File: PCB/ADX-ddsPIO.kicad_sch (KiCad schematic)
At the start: 72 parts, among them J1 Conn_Coaxial, J2 +12V, Q1 BS170, Q2 BS170, Q3 BS170, Q5 BS170, U1 L7805, U2 74LS244, U4 CD2003GB_GP

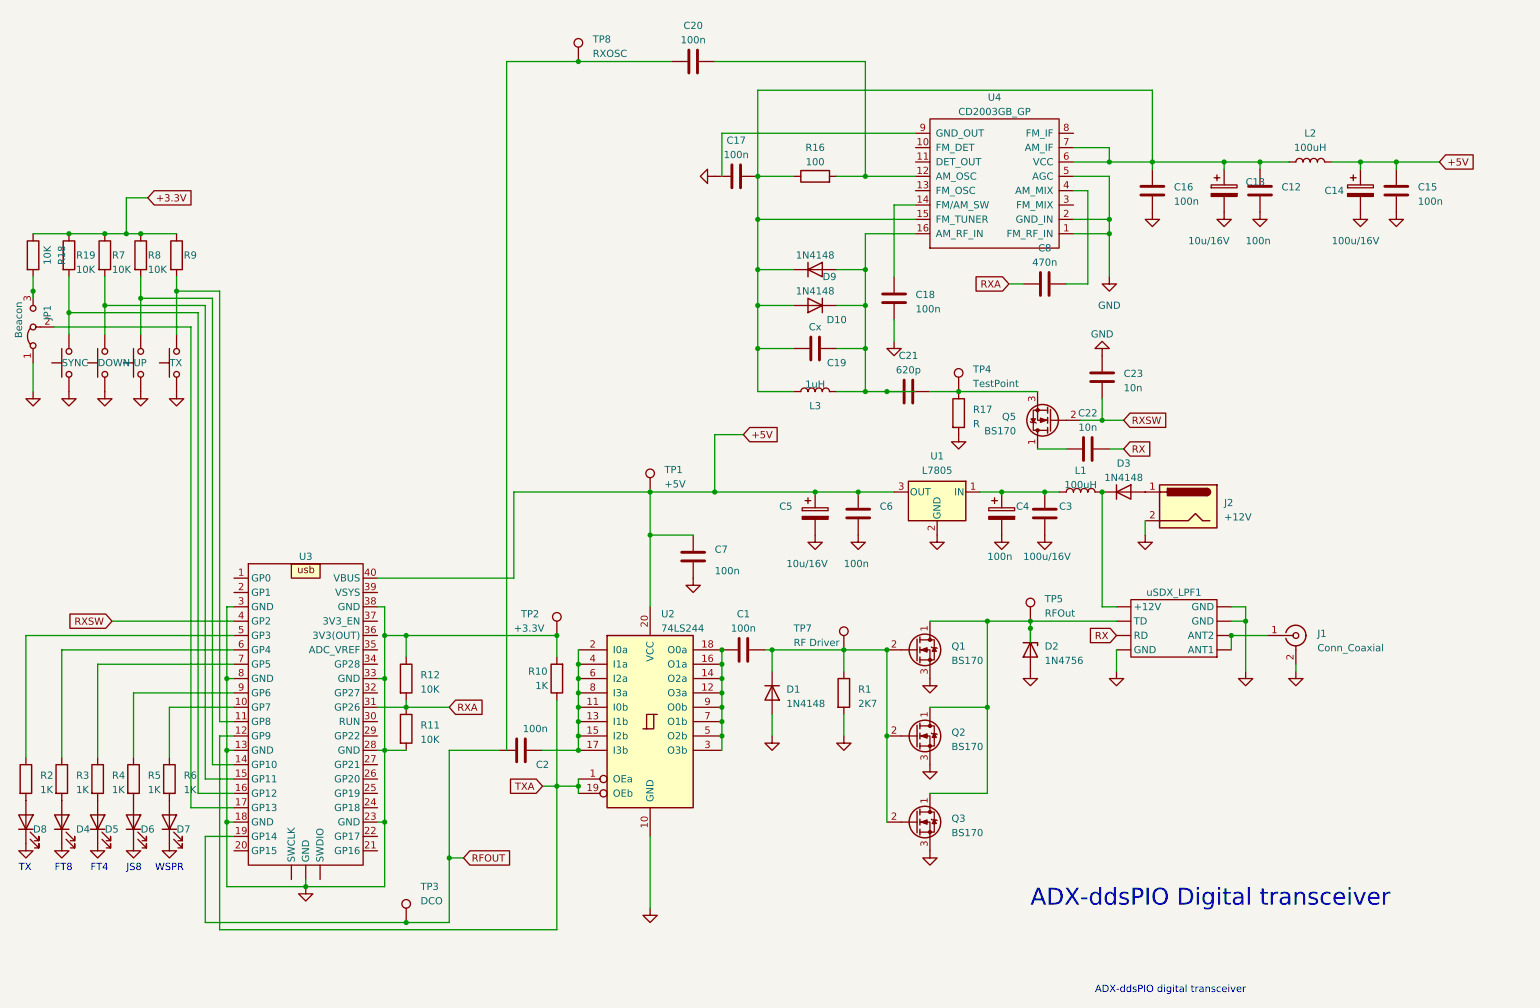
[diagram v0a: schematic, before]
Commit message: ADX-ddsPIO_V1.2
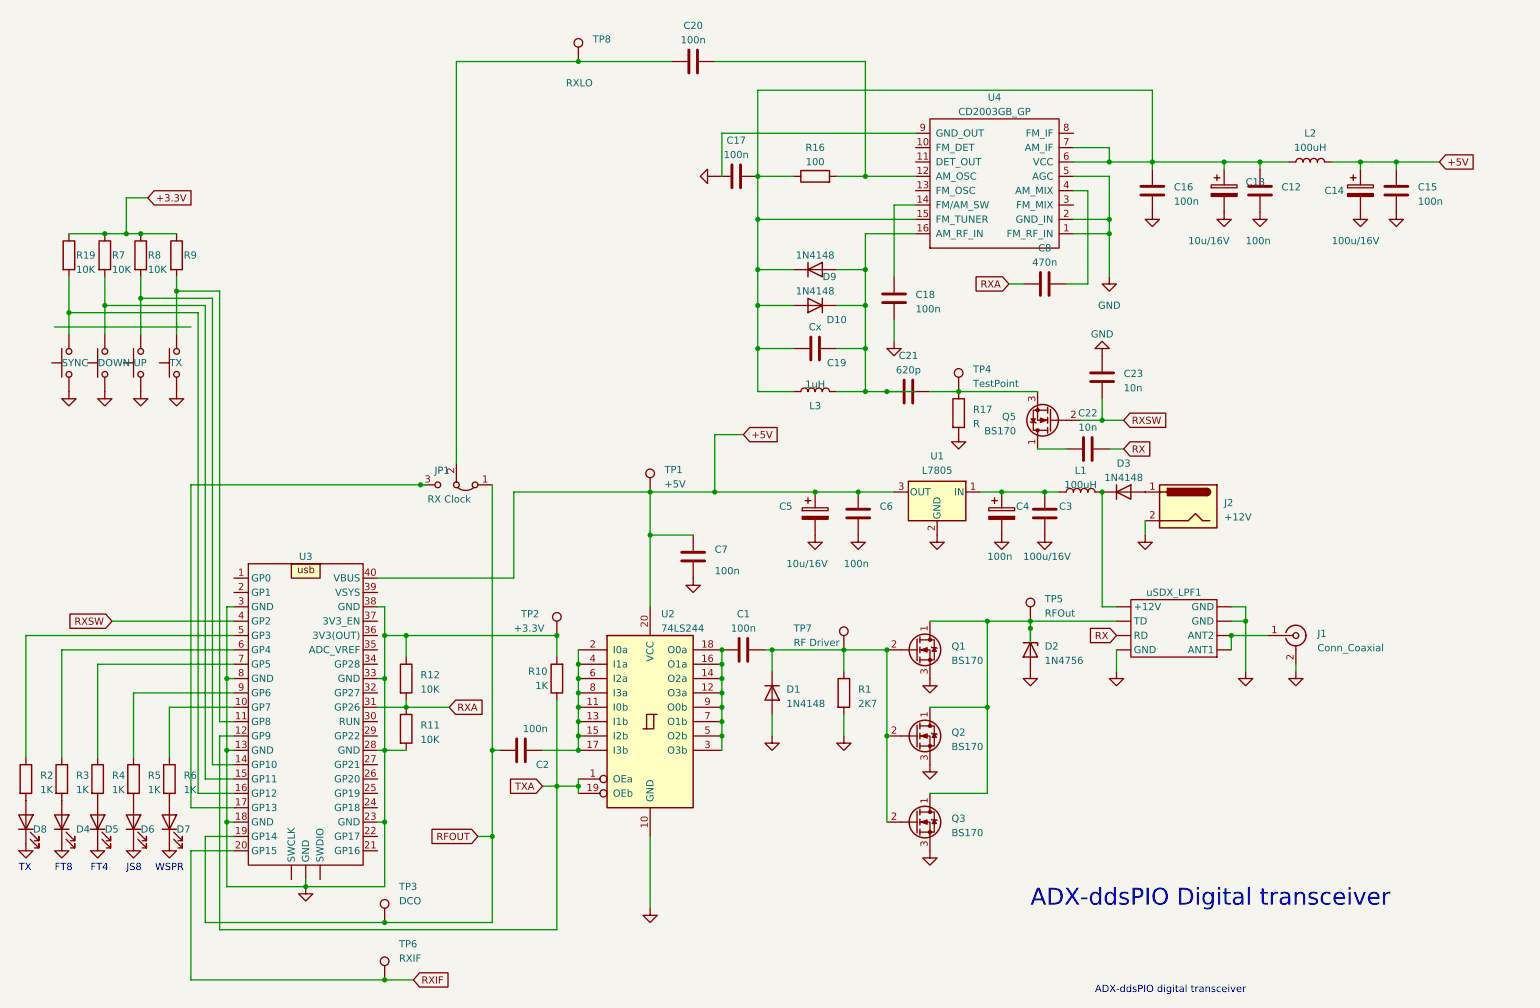
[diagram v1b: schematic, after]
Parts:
- removed R18: 10K, symbol Device:R
- added TP6: RXIF, symbol Connector:TestPoint
- JP1: value Beacon -> RX Clock
- TP8: value RXOSC -> RXLO
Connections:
- net GND: no longer JP1.1 (A)
- net RFOUT: now also JP1.1 (A)
- net at JP1.2 (C): now also C20.1, TP8.1; no longer U3.17 (GP13)
- net at JP1.3 (B): now also U3.17 (GP13)
- net RXIF: now reaches U3.20 (GP15)
- net RXIF: now also TP6.1
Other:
- moved on the sheet: TP3
